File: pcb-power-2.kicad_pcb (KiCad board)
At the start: 2 copper layers, 53.6 x 53.7 mm, 18 parts, among them J1 Conn_01x07_Socket, J12 Conn_01x02_Socket, J2 Conn_01x02_Socket, J3 Conn_01x02_Socket, Q2 NMOS, Q4 PMOS, U1 LM1117DT-5.0, U2 IRF7303, U3 LM1117DT-5.0, U4 IRF7104

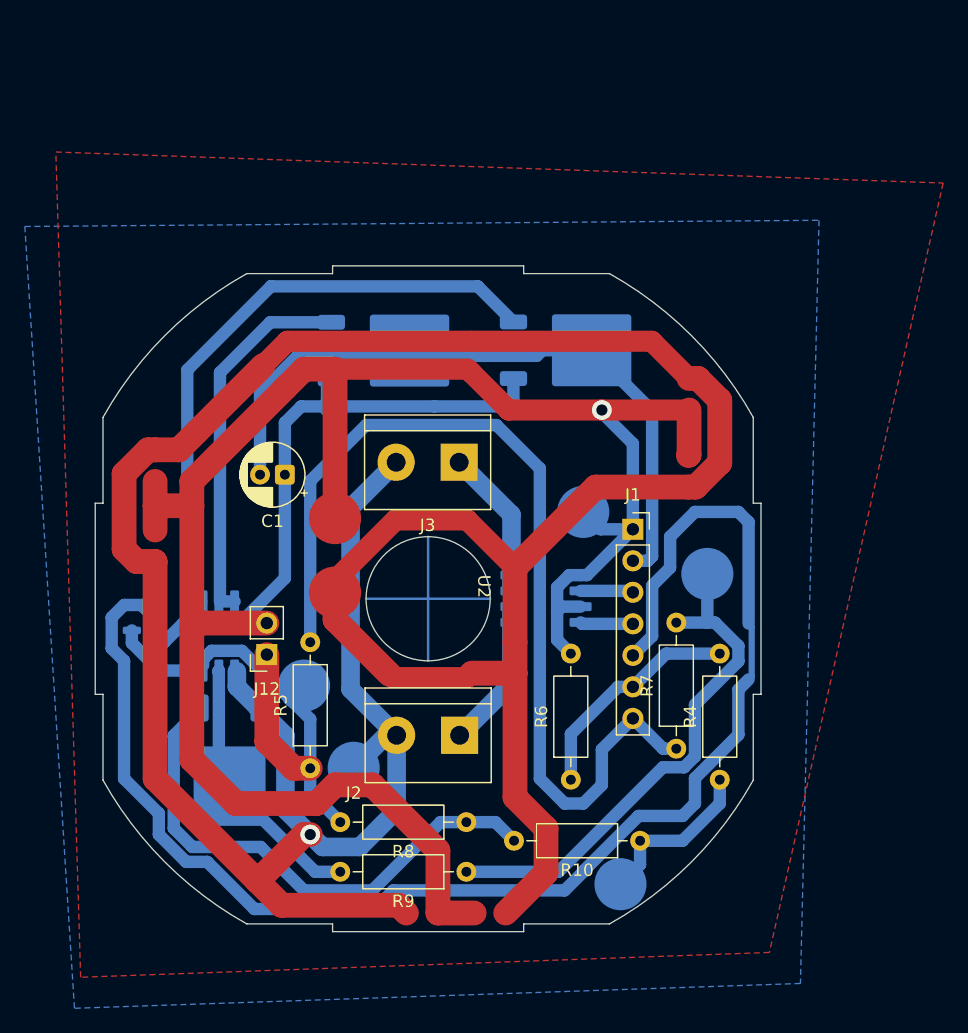
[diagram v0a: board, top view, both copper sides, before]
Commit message: finished pcb design
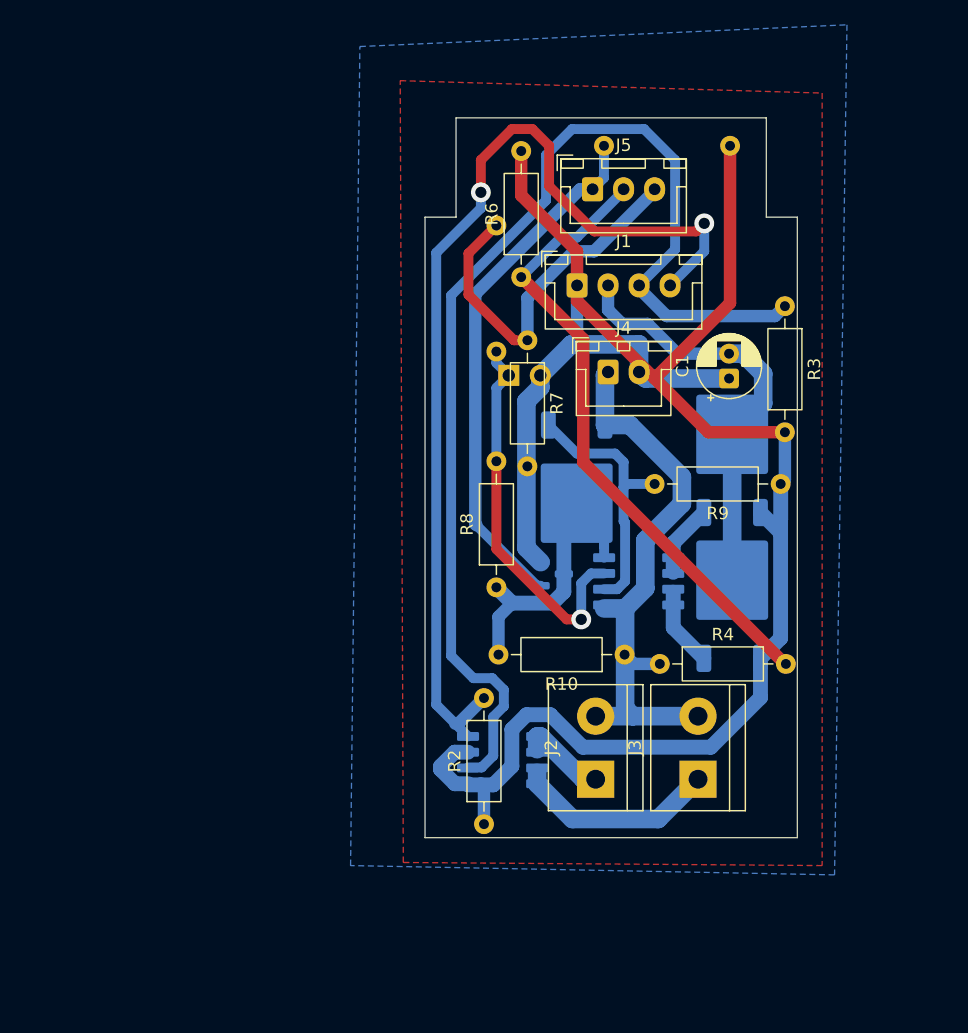
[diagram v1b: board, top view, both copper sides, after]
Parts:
- added J4: Conn_01x02_Socket, Connector_JST:JST_XH_B2B-XH-A_1x02_P2.50mm_Vertical, F.Cu at (138.0, 67.7)
- added J5: Conn_01x03_Socket, Connector_JST:JST_XH_B3B-XH-A_1x03_P2.50mm_Vertical, F.Cu at (136.8, 53.0)
- added R1: 10k, Resistor_THT:R_Axial_DIN0207_L6.3mm_D2.5mm_P10.16mm_Horizontal, B.Cu at (137.7, 49.5)
- added R2: 10k, Resistor_THT:R_Axial_DIN0207_L6.3mm_D2.5mm_P10.16mm_Horizontal, F.Cu at (128.0, 104.2)
- added R3: 10k, Resistor_THT:R_Axial_DIN0207_L6.3mm_D2.5mm_P10.16mm_Horizontal, F.Cu at (152.2, 62.4)
- J1: value Conn_01x07_Socket -> Conn_01x04_Socket; footprint Connector_PinSocket_2.54mm:PinSocket_1x07_P2.54mm_Vertical -> Connector_JST:JST_XH_B4B-XH-A_1x04_P2.50mm_Vertical
- J12, R5: moved to B.Cu
- moved R6 40.7 mm to (131.0, 60.1)
- moved R9 40.2 mm to (151.9, 76.8)
- moved R5 36.8 mm to (129.0, 66.1)
- moved C1 36.6 mm to (147.8, 68.2), turned to 90 degrees
- moved Q4 36.1 mm to (135.5, 77.0)
- moved R7 35.0 mm to (131.5, 65.2), turned to -90 degrees
- moved U4 34.7 mm to (140.5, 84.6), turned to 90 degrees
- moved U1 33.7 mm to (148.0, 85.8), turned to 90 degrees
- moved Q2 33.3 mm to (133.5, 84.0), turned to 0 degrees
- moved J3 32.0 mm to (145.2, 100.5), turned to 90 degrees
- moved J12 29.8 mm to (130.0, 68.0), turned to -90 degrees
- moved J1 20.2 mm to (135.5, 60.8)
- moved R8 19.1 mm to (129.0, 85.1), turned to 90 degrees
- moved R10 15.1 mm to (139.3, 90.5)
- moved U3 14.9 mm to (148.0, 74.0), turned to 90 degrees
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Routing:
- net VCC main: track 278.1 -> 46.8 mm, vias 1 -> 0
- net GND: track 257.8 -> 159.7 mm, vias 1 -> 0
- net PYRO 1: track 4.26 -> 93.9 mm
- net PYRO 2: track 4.26 -> 82.9 mm, vias 0 -> 2
- net signal: track 115.7 -> 42.7 mm
- net PROBE sec: track 77.2 -> 30.1 mm
- net Net-(U3-VI): track 50.1 -> 5.84 mm
- net PROBE main: track 18.4 -> 51.2 mm
- net MODE: track 53.2 -> 23.8 mm
- net Net-(U1-VI): track 30.3 -> 6.35 mm
- net +3.3V: track 55.0 -> 34.3 mm
- net Net-(J3-Pin_1): track 12.1 -> 16.4 mm
- net Net-(J2-Pin_1): track 11.7 -> 7.57 mm
- net VCC secondary: track 32.4 -> 31.0 mm, vias 0 -> 1
- net Net-(Q4-D): track 22.4 -> 21.5 mm
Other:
- board size 53.6 x 53.7 mm -> 30 x 58 mm
